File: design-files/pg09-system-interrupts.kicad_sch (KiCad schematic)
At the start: 32 parts, among them U401 W65C21, U402 74HC04, U403 74HC04, U404 74HC04, U405 74HC00, U406 74HC00, U407 74HC00, U408 74HC00, U409 74HC148, U410 74HC148, U411 GAL22V10, U412 74AHC138, U413 74AHC374, U414 74AHC374

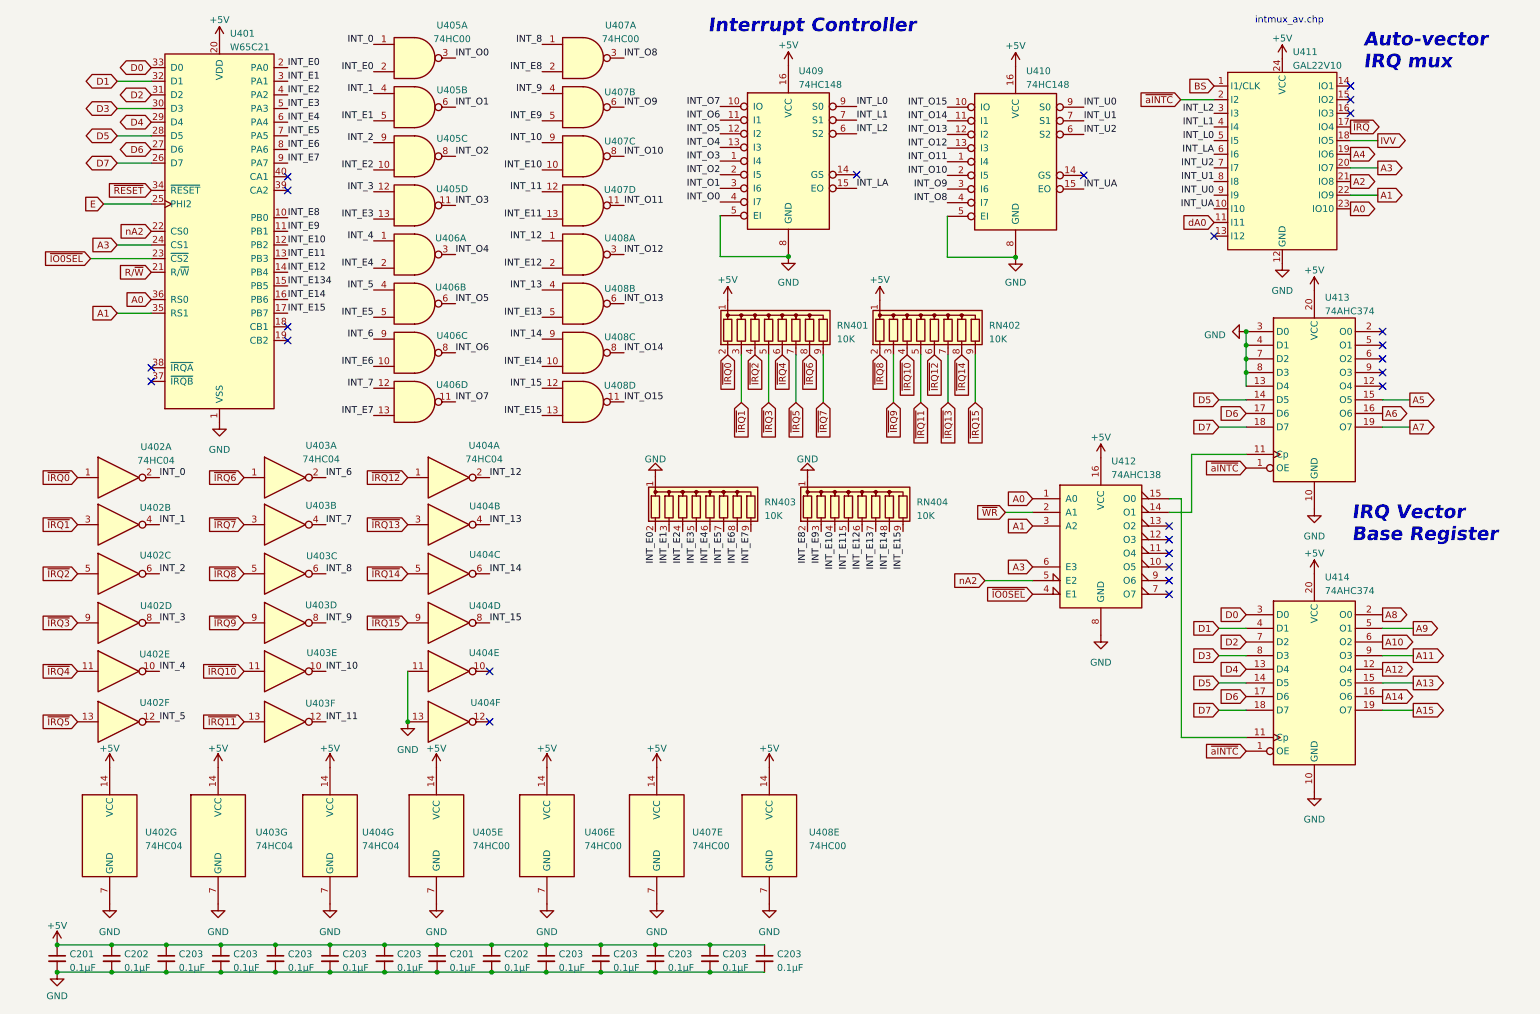
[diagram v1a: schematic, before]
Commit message: Move the 74AHC05 from the UART sheet to the INTC sheet.
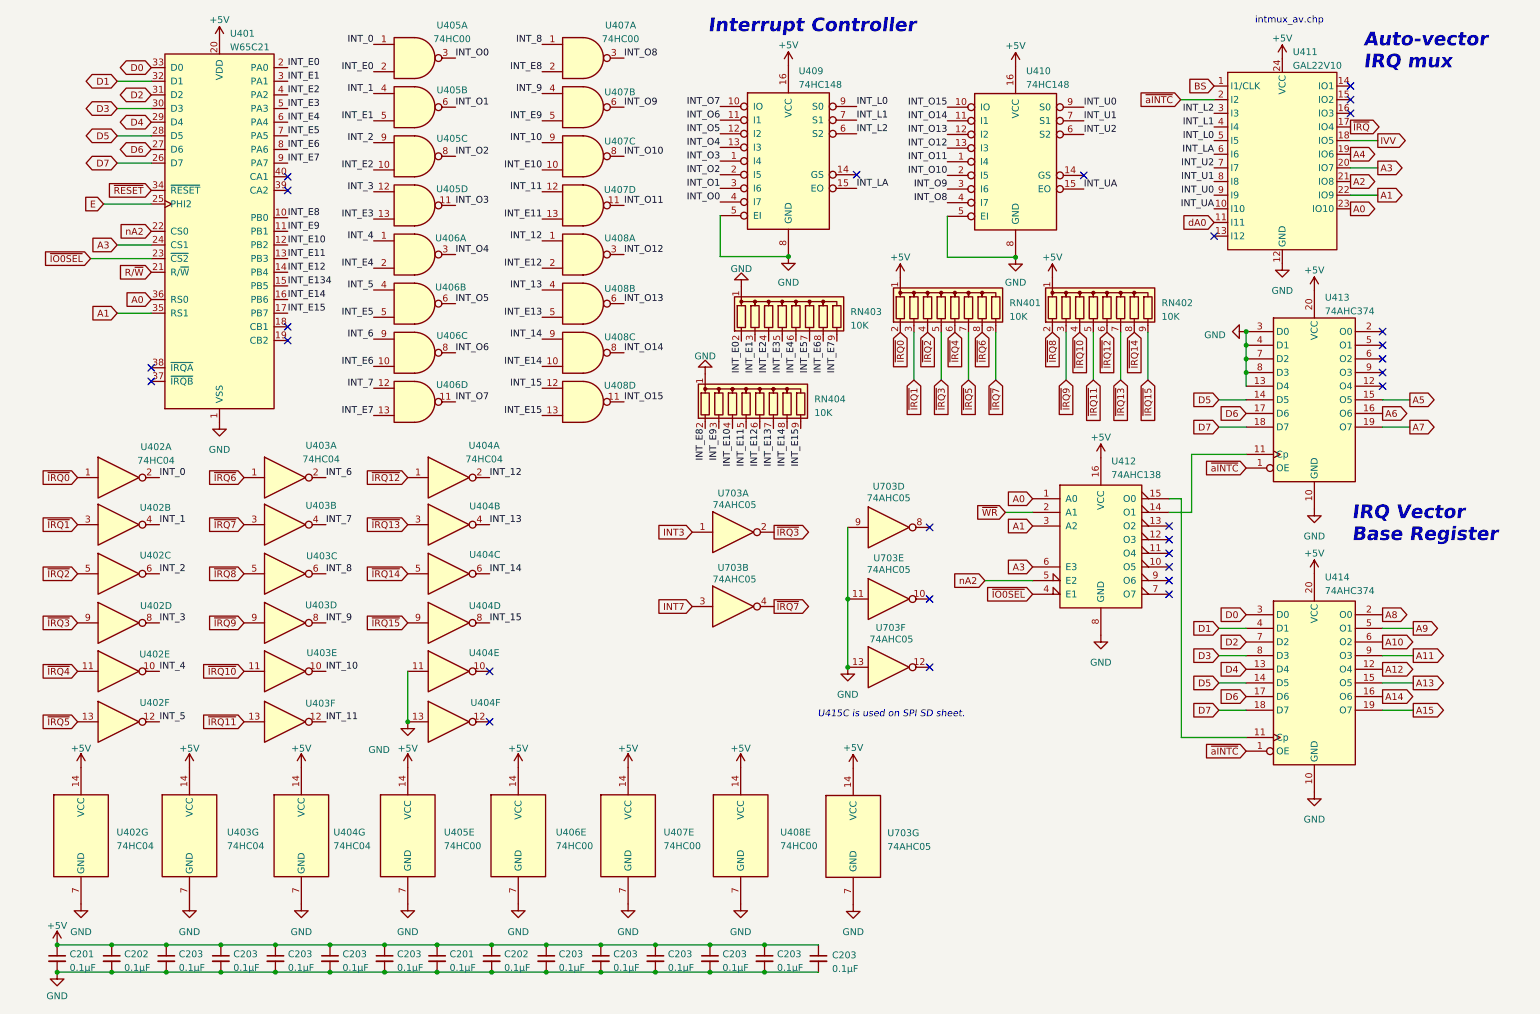
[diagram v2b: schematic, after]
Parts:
- added C203: 0.1µF, Capacitor_THT:C_Disc_D3.8mm_W2.6mm_P2.50mm, symbol Device:C_Small
- added U703: 74AHC05, Package_DIP:DIP-14_W7.62mm_Socket, symbol 74xx:74LS05
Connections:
- net +5V: now also C203.1, U703.14 (VCC)
- net GND: now also C203.2, U703.11, U703.13, U703.7 (GND), U703.9
- net ~{IRQ3}: now also U703.2
- net ~{IRQ7}: now also U703.4
- new net INT3: U703.1
- new net INT7: U703.3
- no-connect marks 25 -> 28
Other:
- note added: "U415C is used on SPI SD sheet."
- moved on the sheet: RN401, RN402, RN403, RN404, U402G, U403G, U404G, U405E, U406E, U407E, U408E
